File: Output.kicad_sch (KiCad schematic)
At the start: 4 parts, among them J6 +3.3V, J7 +6V, J8 +3.3V, J9 +6V

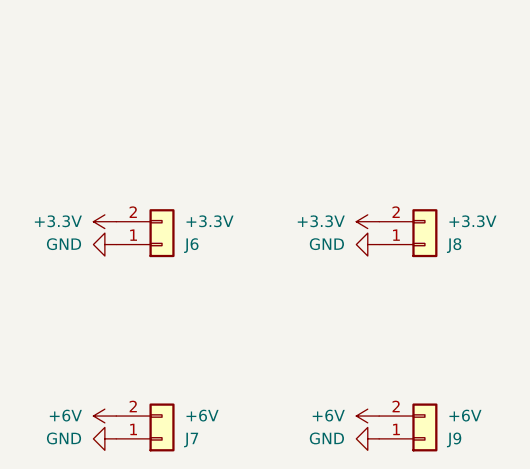
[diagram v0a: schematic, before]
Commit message: update sch
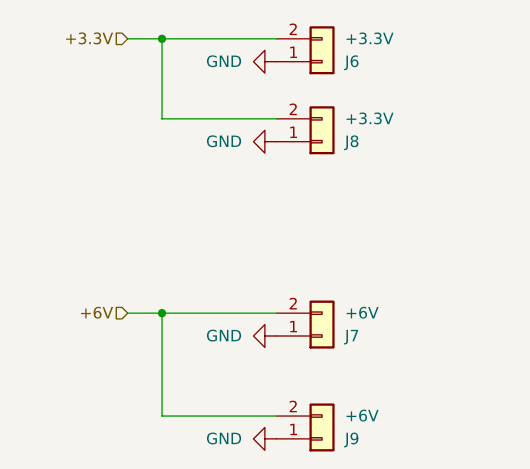
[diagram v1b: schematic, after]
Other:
- moved on the sheet: J6, J7, J8, J9
